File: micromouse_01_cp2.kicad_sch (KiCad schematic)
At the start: 28 parts, among them IC2 MPU-6500, IC3 AS5047P-ATSM, IC4 AS5047P-ATSM, IC5 DRV8835DSSR, M1 MK06-4.5, M2 MK06-4.5, U9 ESP32-S3-PICO-1-N8R2

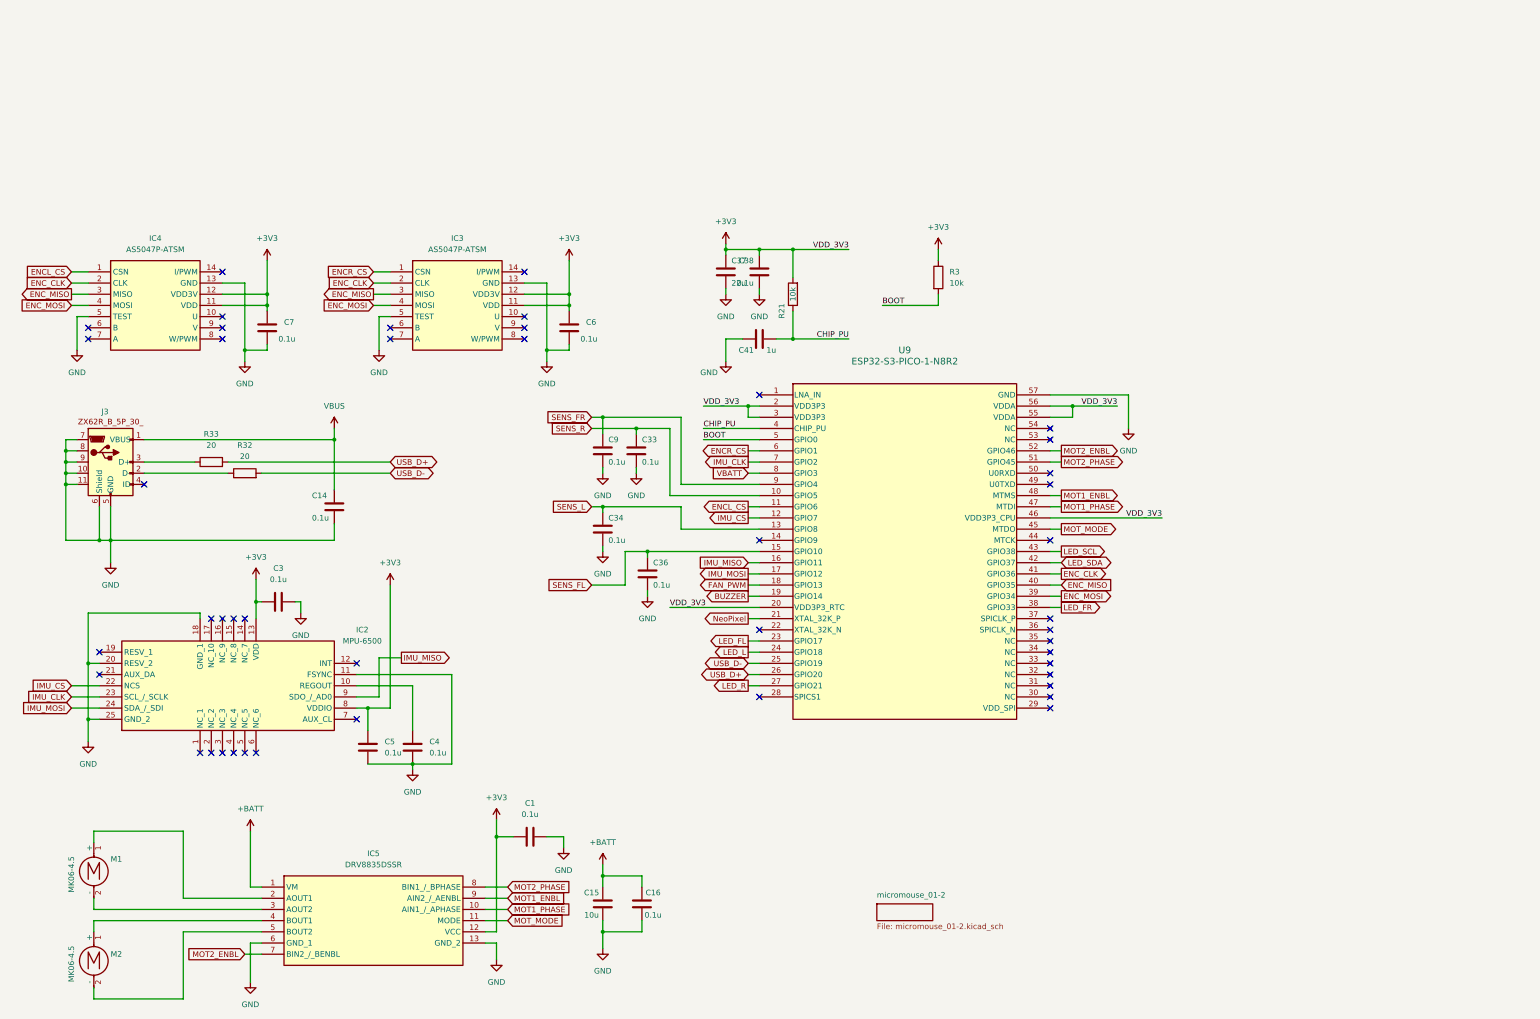
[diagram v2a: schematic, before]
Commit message: エンコーダ基板変更前コミット
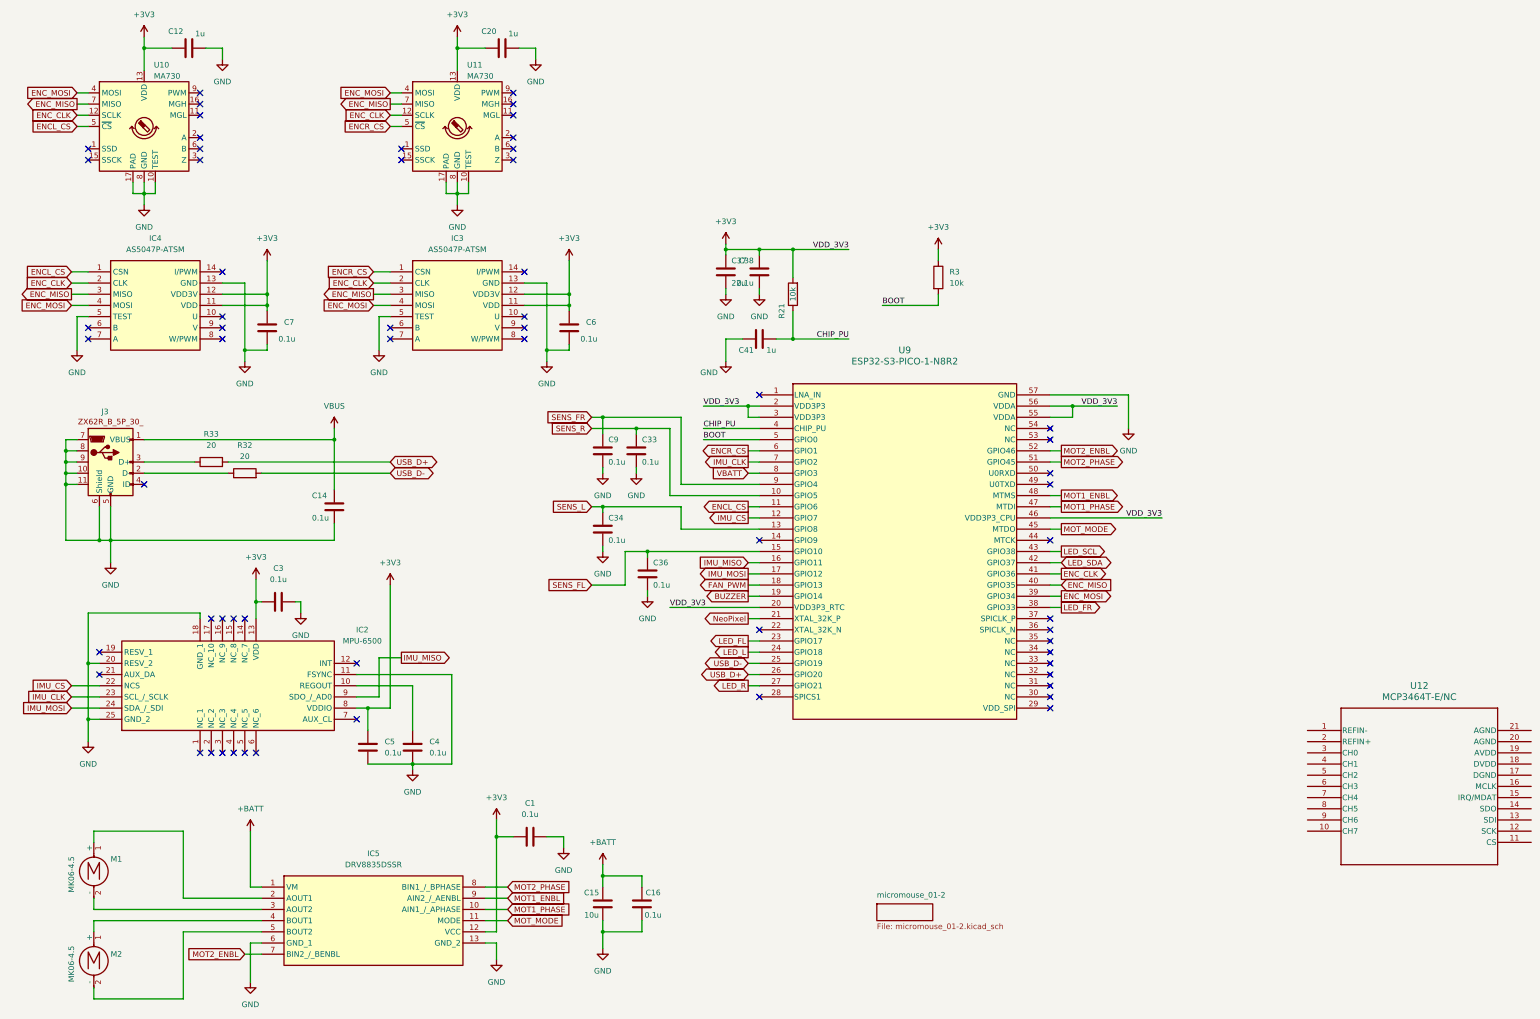
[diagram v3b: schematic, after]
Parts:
- added C12, C20: 1u, Capacitor_SMD:C_0402_1005Metric, symbol Device:C
- added U10, U11: MA730, Package_DFN_QFN:QFN-16-1EP_3x3mm_P0.5mm_EP1.75x1.75mm, symbol Sensor_Magnetic:MA730
- added U12: MCP3464T-E/NC, UQFN20_NC_MCH, symbol 2024-03-13_05-36-02:MCP3464T-E_NC
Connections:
- net +3V3: now also C12.1, C20.1, U10.13 (VDD), U11.13 (VDD)
- net ENCL_CS: now also U10.5 (~{CS})
- net ENCR_CS: now also U11.5 (~{CS})
- net ENC_CLK: now also U10.12 (SCLK), U11.12 (SCLK)
- net ENC_MISO: now also U10.7 (MISO), U11.7 (MISO)
- net ENC_MOSI: now also U10.4 (MOSI), U11.4 (MOSI)
- net GND: now also C12.2, C20.2, U10.10 (TEST), U10.17 (PAD), U10.8 (GND), U11.10 (TEST), U11.17 (PAD), U11.8 (GND)
- no-connect marks 45 -> 61

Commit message: とりあえず回路図完成
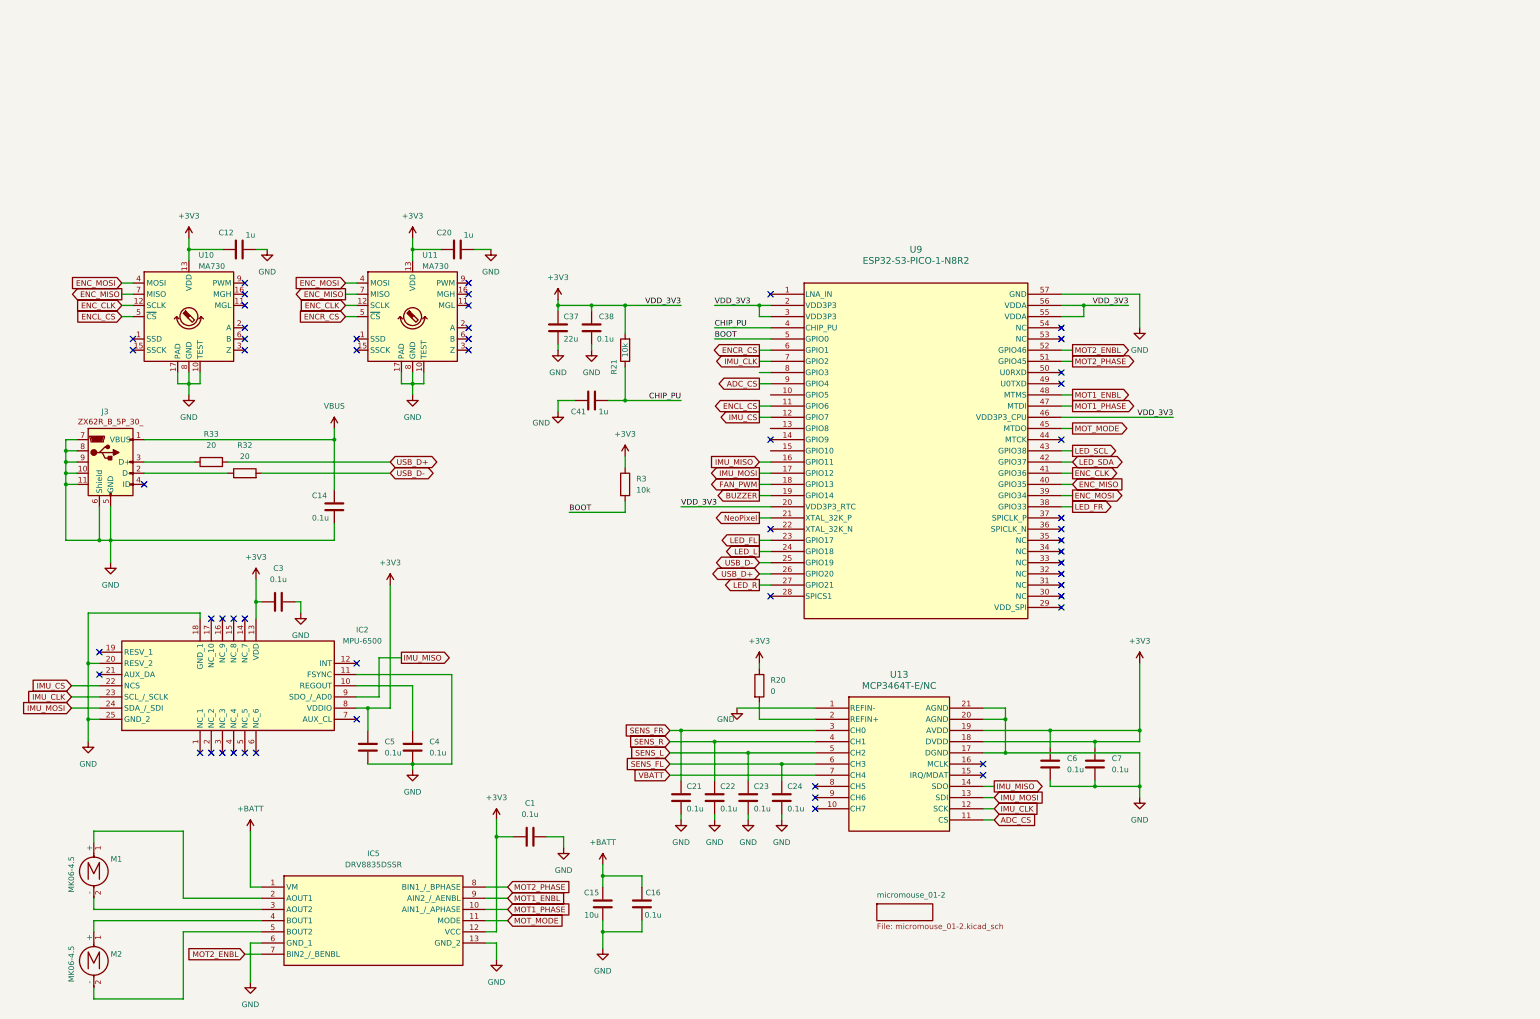
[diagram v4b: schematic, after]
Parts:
- removed C33, C34, C36, C9: 0.1u, Capacitor_SMD:C_0402_1005Metric, symbol Device:C
- removed IC3, IC4: AS5047P-ATSM, footprints:SOP65P640X120-14N, symbol AS5047P-ATSM:AS5047P-ATSM
- removed U12: MCP3464T-E/NC, UQFN20_NC_MCH, symbol 2024-03-13_05-36-02:MCP3464T-E_NC
- added C21, C22, C23, C24: 0.1u, Capacitor_SMD:C_0402_1005Metric, symbol Device:C
- added R20: 0, symbol Device:R
- added U13: MCP3464T-E/NC, UQFN20_NC_MCH, symbol 2024-03-13_05-36-02:MCP3464T-E_NC
- C6, C7: footprint Capacitor_SMD:C_0402_1005Metric -> (none)
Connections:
- net +3V3: now also R20.1, U13.18 (DVDD), U13.19 (AVDD)
- net GND: now also C21.2, C22.2, C23.2, C24.2, U13.1 (REFIN-), U13.17 (DGND), U13.20 (AGND), U13.21 (AGND)
- net IMU_CLK: now also U13.12 (SCK)
- net IMU_MISO: now also U13.14 (SDO)
- net IMU_MOSI: now also U13.13 (SDI)
- net SENS_FL: now also C24.1, U13.6 (CH3); no longer U9.15 (GPIO10)
- net SENS_FR: now also C21.1, U13.3 (CH0); no longer U9.9 (GPIO4)
- net SENS_L: now also C23.1, U13.5 (CH2); no longer U9.13 (GPIO8)
- net SENS_R: now also C22.1, U13.4 (CH1); no longer U9.10 (GPIO5)
- net VBATT: now also U13.7 (CH4); no longer U9.8 (GPIO3)
- new net: R20.2, U13.2 (REFIN+)
- new net ADC_CS: U13.11 (CS), U9.9 (GPIO4)
- no-connect marks 61 -> 54
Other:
- moved on the sheet: C12, C20, C37, C38, C41, R21, R3, U10, U11, U9

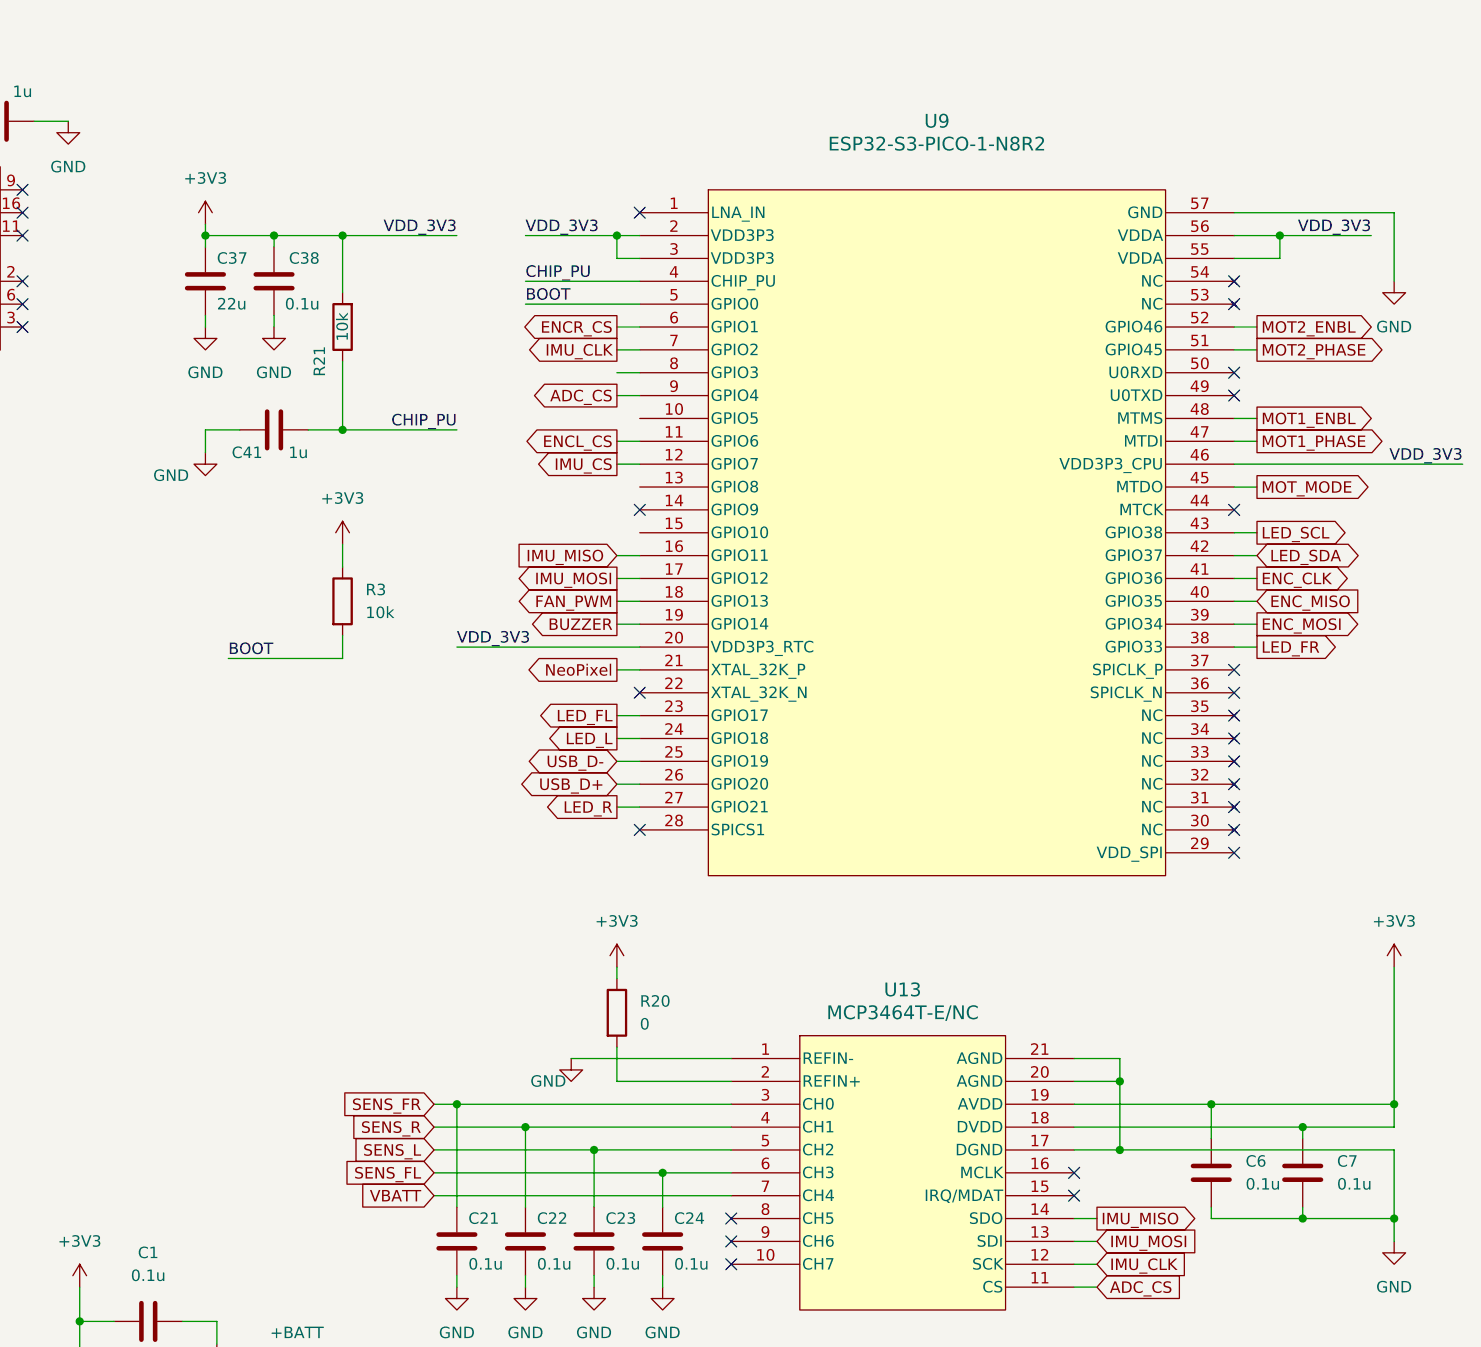
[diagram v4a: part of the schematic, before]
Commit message: パターン配線中
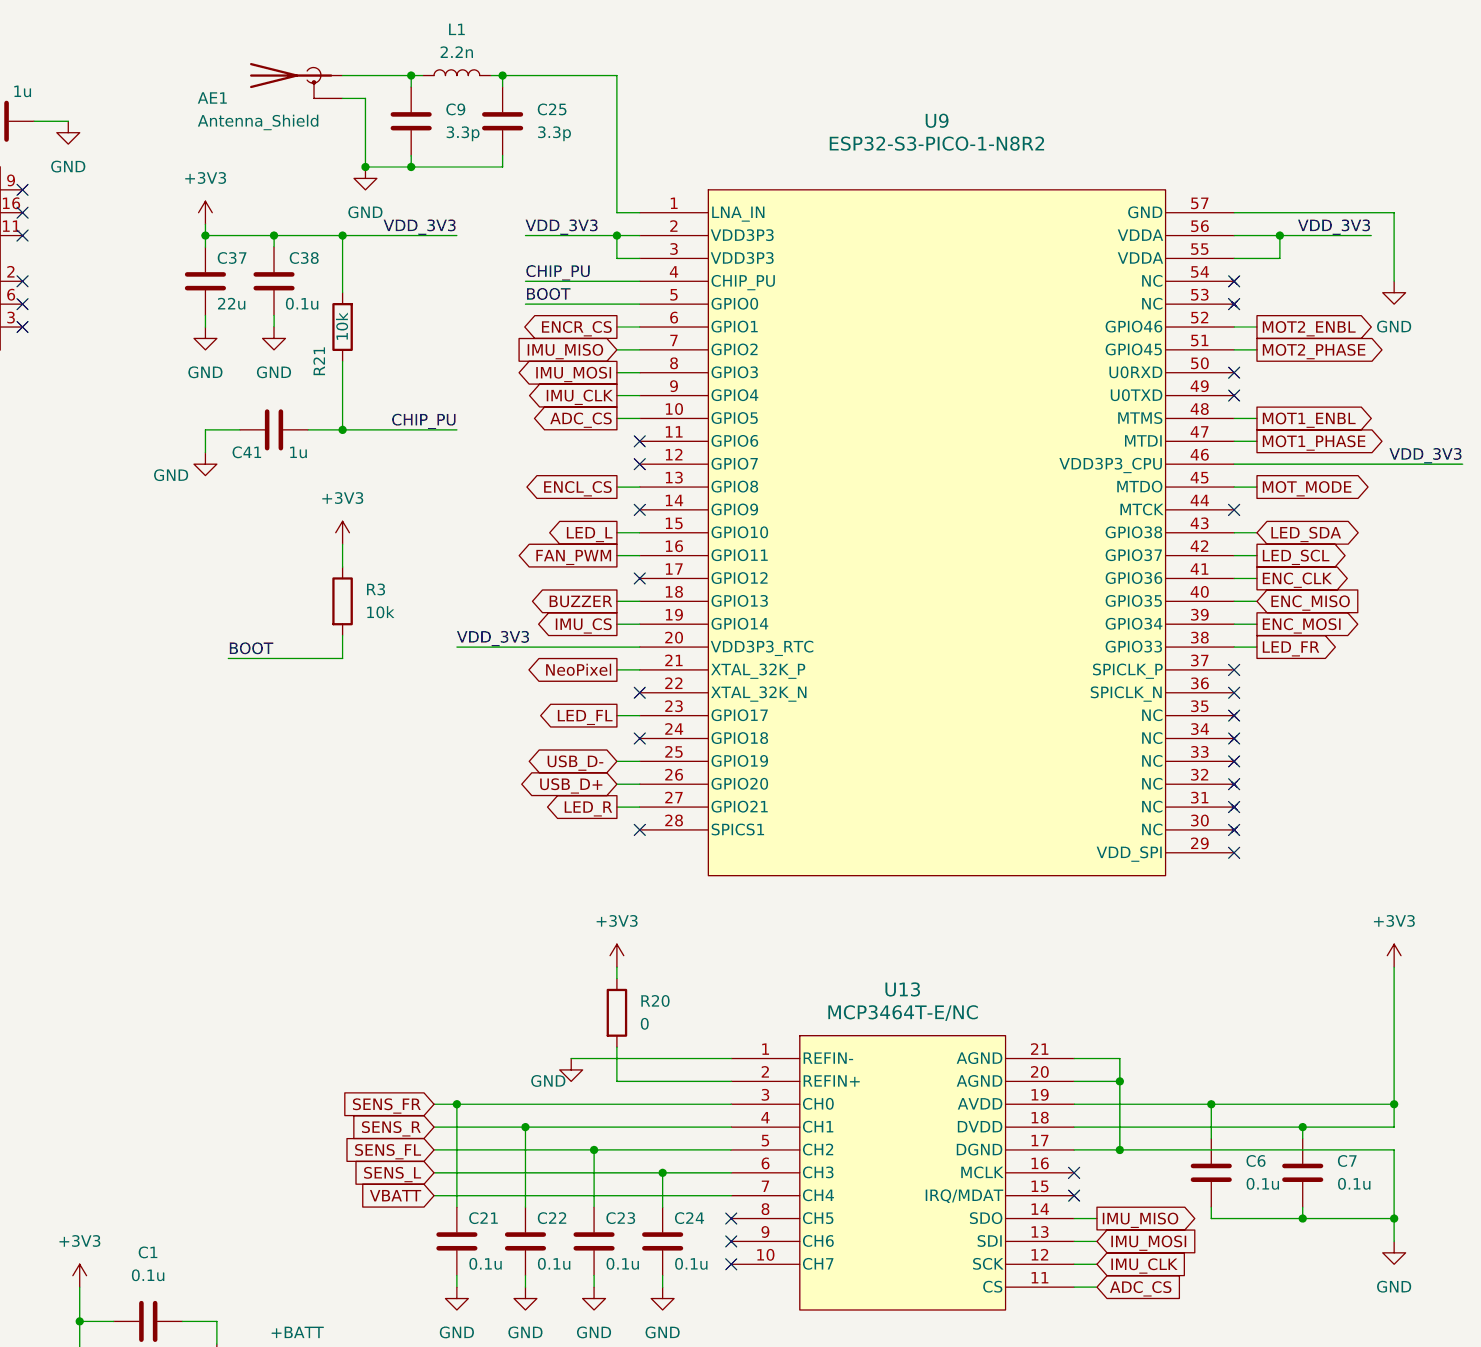
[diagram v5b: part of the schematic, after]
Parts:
- added AE1: Antenna_Shield, RF_Antenna:Texas_SWRA117D_2.4GHz_Right, symbol Device:Antenna_Shield
- added C25, C9: 3.3p, Capacitor_SMD:C_0402_1005Metric, symbol Device:C
- added L1: 2.2n, Inductor_SMD:L_0402_1005Metric, symbol Device:L
- C6, C7: footprint (none) -> Capacitor_SMD:C_0402_1005Metric
- R20: footprint (none) -> Resistor_SMD:R_0402_1005Metric
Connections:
- net ADC_CS: now also U9.10 (GPIO5); no longer U9.9 (GPIO4)
- net BUZZER: now also U9.18 (GPIO13); no longer U9.19 (GPIO14)
- net ENCL_CS: now also U9.13 (GPIO8); no longer U9.11 (GPIO6)
- net FAN_PWM: now also U9.16 (GPIO11); no longer U9.18 (GPIO13)
- net GND: now also AE1.2 (Shield), C25.2, C9.2
- net IMU_CLK: now also U9.9 (GPIO4); no longer U9.7 (GPIO2)
- net IMU_CS: now also U9.19 (GPIO14); no longer U9.12 (GPIO7)
- net IMU_MISO: now also U9.7 (GPIO2); no longer U9.16 (GPIO11)
- net IMU_MOSI: now also U9.8 (GPIO3); no longer U9.17 (GPIO12)
- net LED_L: now also U9.15 (GPIO10); no longer U9.24 (GPIO18)
- net LED_SCL: now also U9.42 (GPIO37); no longer U9.43 (GPIO38)
- net LED_SDA: now also U9.43 (GPIO38); no longer U9.42 (GPIO37)
- net SENS_FL: now also C23.1, U13.5 (CH2); no longer C24.1, U13.6 (CH3)
- net SENS_L: now also C24.1, U13.6 (CH3); no longer C23.1, U13.5 (CH2)
- net at U9.1 (LNA_IN): now also C25.1, L1.2
- new net: AE1.1 (A), C9.1, L1.1
- no-connect marks 54 -> 57
